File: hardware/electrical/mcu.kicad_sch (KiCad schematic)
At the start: 38 parts, among them J2 STDC14, SW1 SW_Push, SW2 SW_Push, U8 STM32F446VET6, Y1 24MHz, Y2 32.768kHz

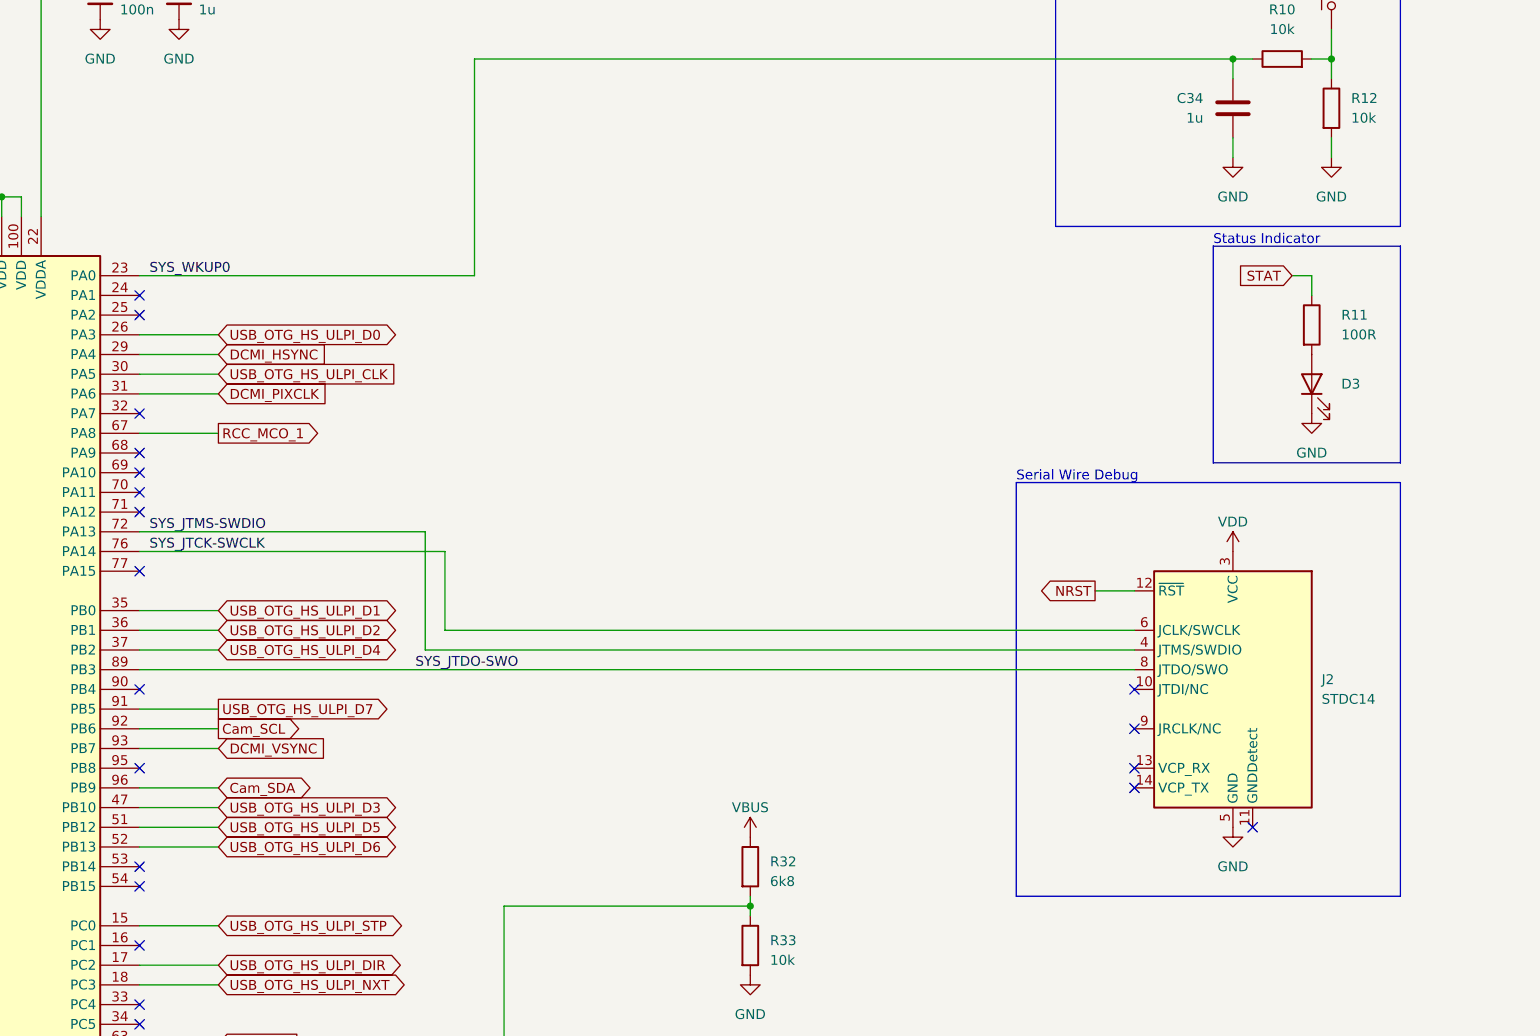
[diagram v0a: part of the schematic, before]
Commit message: Component selection
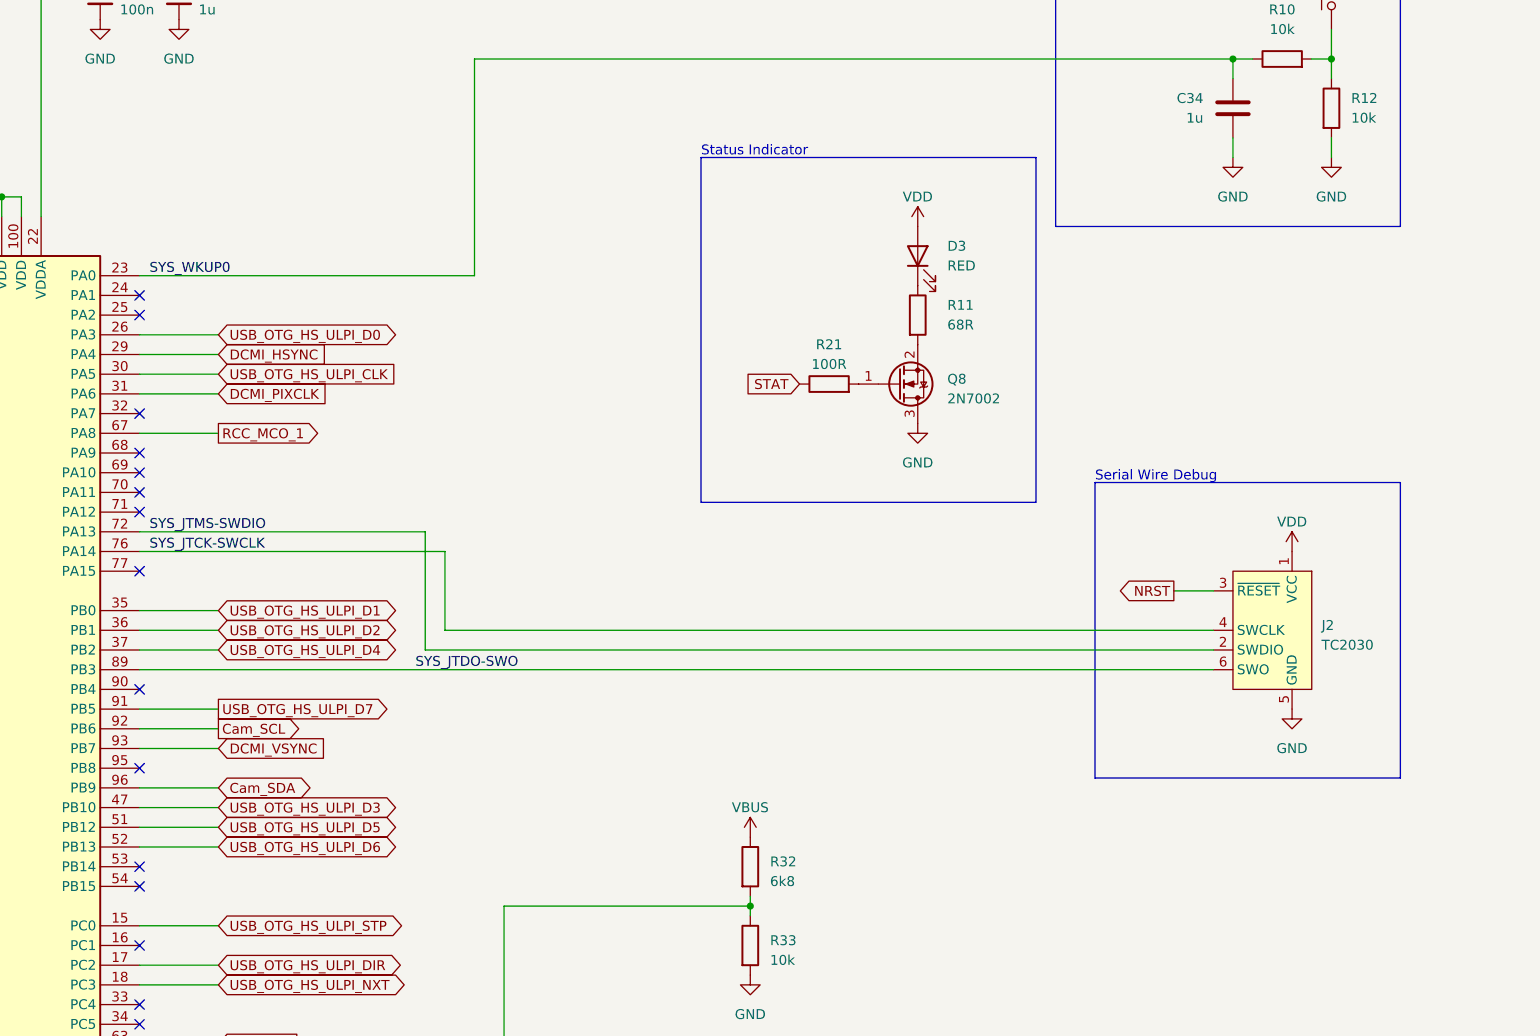
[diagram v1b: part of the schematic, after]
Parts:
- removed J2: STDC14, symbol Connector:Conn_ST_STDC14
- added J2: TC2030, Connector:Tag-Connect_TC2030-IDC-FP_2x03_P1.27mm_Vertical, symbol Connector:Conn_ARM_SWD_TagConnect_TC2030
- added Q8: 2N7002, Package_TO_SOT_SMD:SOT-23, symbol Transistor_FET:2N7002
- added R21: 100R, Resistor_SMD:R_0402_1005Metric, symbol Device:R
- C10, C12, C13, C15, C16, C17, C18, C27, C29: footprint (none) -> Capacitor_SMD:C_0402_1005Metric; LCSC Part # (none) -> C1525; Mfr (none) -> Samsung Electro-Mechanics; Mfr. Part # (none) -> CL05B104KO5NNNC
- C11, C14: footprint (none) -> Capacitor_SMD:C_0603_1608Metric; LCSC Part # (none) -> C38523; Mfr (none) -> Samsung Electro-Mechanics; Mfr. Part # (none) -> CL10C120JB8NNNC
- C20, C22: footprint (none) -> Capacitor_SMD:C_0402_1005Metric; LCSC Part # (none) -> C12530; Mfr (none) -> Samsung Electro-Mechanics; Mfr. Part # (none) -> CL05A225MQ5NSNC
- C25, C9: footprint (none) -> Capacitor_SMD:C_0402_1005Metric; LCSC Part # (none) -> C23733; Mfr (none) -> Samsung Electro-Mechanics; Mfr. Part # (none) -> CL05A475MP5NRNC
- C31, C34: footprint (none) -> Capacitor_SMD:C_0402_1005Metric; LCSC Part # (none) -> C52923; Mfr (none) -> Samsung Electro-Mechanics; Mfr. Part # (none) -> CL05A105KA5NQNC
- C32, C33: footprint (none) -> Capacitor_SMD:C_0603_1608Metric; LCSC Part # (none) -> C1644; Mfr (none) -> Samsung Electro-Mechanics; Mfr. Part # (none) -> CL10C150JB8NNNC
- D3: value LED -> RED; LCSC Part # (none) -> C131288; Mfr (none) -> Everlight Elec; Mfr. Part # (none) -> 12-21SURC/S530-A3/TR8
- JP1: now left out of the parts list
- R10, R12, R33, R7: footprint (none) -> Resistor_SMD:R_0402_1005Metric; LCSC Part # (none) -> C25744; Mfr (none) -> UNI-ROYAL(Uniroyal Elec); Mfr. Part # (none) -> 0402WGF1002TCE
- R11: value 100R -> 68R; footprint (none) -> Resistor_SMD:R_0603_1608Metric; LCSC Part # (none) -> C27592; Mfr (none) -> UNI-ROYAL(Uniroyal Elec); Mfr. Part # (none) -> 0603WAF680JT5E
- R32: footprint (none) -> Resistor_SMD:R_0402_1005Metric; LCSC Part # (none) -> C25917; Mfr (none) -> UNI-ROYAL(Uniroyal Elec); Mfr. Part # (none) -> 0402WGF6801TCE
- R4, R5, R8, R9: footprint (none) -> Resistor_SMD:R_0603_1608Metric_Pad0.98x0.95mm_HandSolder; LCSC Part # (none) -> C21189; Mfr (none) -> UNI-ROYAL(Uniroyal Elec); Mfr. Part # (none) -> 0603WAF0000T5E
- R6: footprint (none) -> Resistor_SMD:R_0402_1005Metric; LCSC Part # (none) -> C25105; Mfr (none) -> UNI-ROYAL(Uniroyal Elec); Mfr. Part # (none) -> 0402WGF330JTCE
- SW1: value SW_Push -> TS-1187A-B-A-B; LCSC Part # (none) -> C318884; Mfr (none) -> XKB Connectivity; Mfr. Part # (none) -> TS-1187A-B-A-B
- SW2: value SW_Push -> EVQP7C01K; LCSC Part # (none) -> C528965; Mfr (none) -> PANASONIC; Mfr. Part # (none) -> EVQP7C01K
- U8: LCSC Part # (none) -> C91929; Mfr (none) -> STMicroelectronics; Mfr. Part # (none) -> STM32F446VET6
- Y1: footprint (none) -> Crystal:Crystal_SMD_SeikoEpson_TSX3225-4Pin_3.2x2.5mm; LCSC Part # (none) -> C255917; Mfr (none) -> Seiko Epson; Mfr. Part # (none) -> X1E0000210129
- Y2: footprint (none) -> Crystal:Crystal_SMD_3215-2Pin_3.2x1.5mm; LCSC Part # (none) -> C32346; Mfr (none) -> Seiko Epson; Mfr. Part # (none) -> Q13FC1350000400
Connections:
- net GND: now also J2.5 (GND), Q8.3 (D); no longer D3.1 (K)
- net NRST: now also J2.3 (~{RESET})
- net STAT: now also R21.1; no longer R11.1
- net SYS_JTCK-SWCLK: now also J2.4 (SWCLK)
- net SYS_JTDO-SWO: now also J2.6 (SWO)
- net SYS_JTMS-SWDIO: now also J2.2 (SWDIO)
- net VDD: now also D3.2 (A), J2.1 (VCC)
- net at R11.2: now also Q8.2 (S); no longer D3.2 (A)
- new net: D3.1 (K), R11.1
- new net: Q8.1 (G), R21.2
- no-connect marks 45 -> 40
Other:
- moved on the sheet: D3, R11
